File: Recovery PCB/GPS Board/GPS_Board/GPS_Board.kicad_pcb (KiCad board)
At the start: 2 copper layers, 85.7 x 50.8 mm, 11 parts, among them J1 XT30-M, J2 XT30-M, U1 Teensy4.1

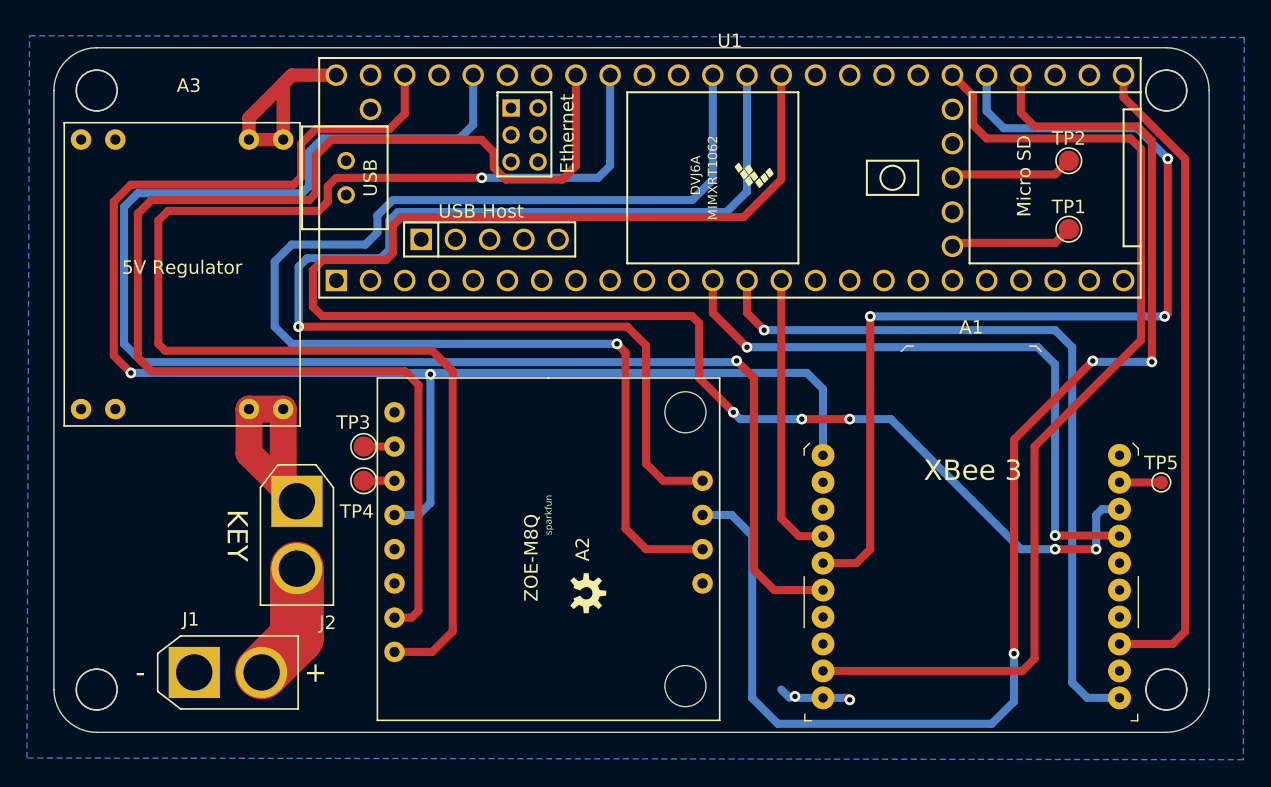
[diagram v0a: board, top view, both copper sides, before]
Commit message: Initial Board Layout
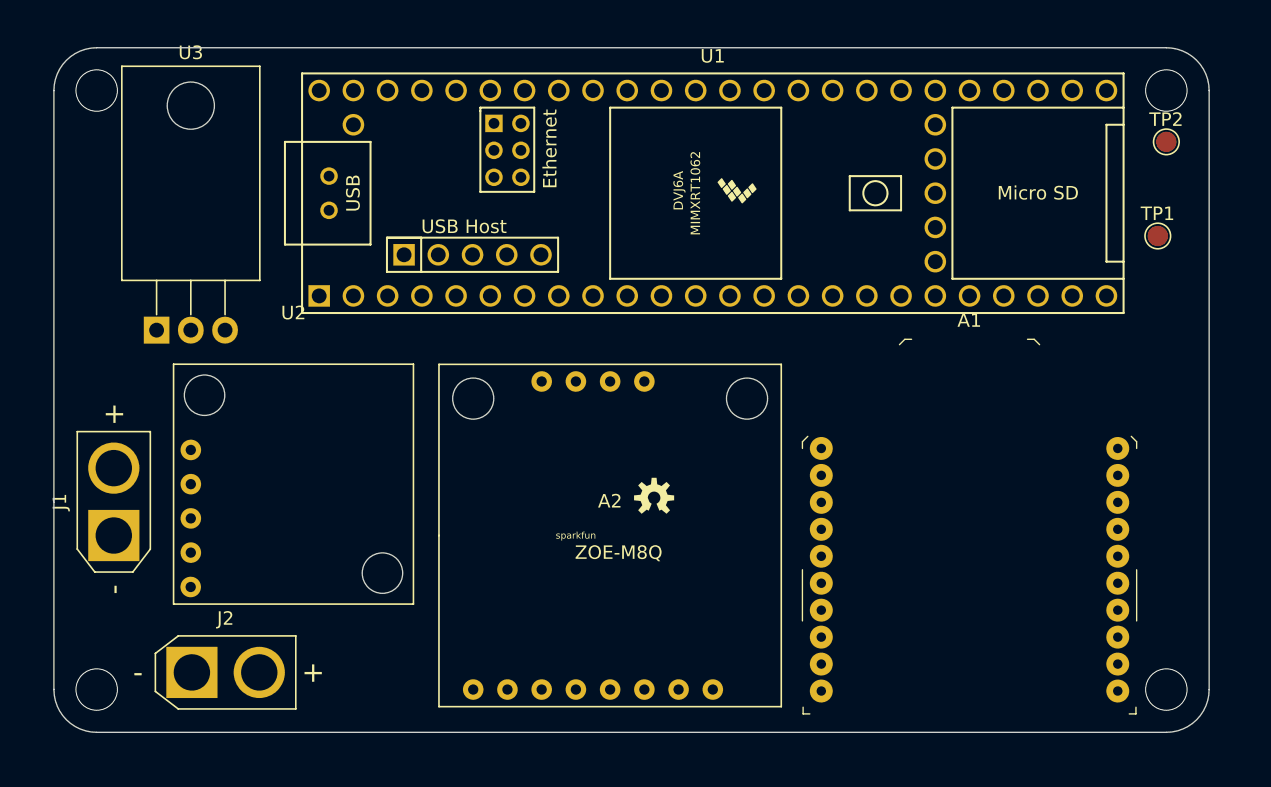
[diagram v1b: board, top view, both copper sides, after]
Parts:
- removed A3: Eboot-MP1584EN-5V-Power-Supply, GPS Board:EBOOT-MP1584EN-5N-POWER-SUPPLY
- removed TP3, TP4: TestPoint, TestPoint:TestPoint_Pad_D1.5mm
- removed TP5: TestPoint, TestPoint:TestPoint_Pad_D1.0mm
- added U2: D24V22F5_VoltageRegulator, GPS Board:D24V22F5_VoltageRegulator, F.Cu at (128.9, 92.7)
- added U3: LD1117v33, Package_TO_SOT_THT:TO-220-3_Horizontal_TabDown, F.Cu at (118.7, 81.3)
- moved J2 14.9 mm to (121.4, 106.7), turned to 0 degrees
- moved J1 11.8 mm to (115.6, 96.5), turned to 90 degrees
- moved TP2 7.37 mm to (193.7, 67.3)
- moved TP1 6.62 mm to (193.0, 74.3)
- moved A2 4.68 mm to (152.4, 96.5), turned to 0 degrees
- moved U1 1.71 mm to (160.0, 71.1)
- moved A1 0.52 mm to (179.1, 99.1)
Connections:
- net MOSI renamed /XBee_MOSI
- net Net-(A1-Pad13) renamed /XBEE_SLEEP
- net Net-(A1-Pad17) renamed /XBee_CS
- net Net-(A1-Pad18) renamed /XBee_SCK
- net Net-(A1-Pad4) renamed /XBee_MISO
- net Net-(A1-Pad6) renamed /XBee_PWM
- net Net-(A1-Pad9) renamed /XBee_DTR
- net Net-(A2-Pad7) renamed /GPS_SCL
- net Net-(A2-Pad8) renamed /GPS_SDA
- A1 pad 1: Net-(A1-Pad1) -> +3V3
- A1 pad 12: (no net) -> Net-(A1-Pad12)
- A1 pad 14: (no net) -> Net-(A1-Pad14)
- A1 pad 15: (no net) -> Net-(A1-Pad15)
- A1 pad 16: (no net) -> Net-(A1-Pad16)
- A1 pad 19: Net-(A1-Pad19) -> /XBEE_SCL
- A1 pad 2: (no net) -> /XBEE_TX
- A1 pad 20: (no net) -> Net-(A1-Pad20)
- A1 pad 3: (no net) -> /XBEE_RX
- A1 pad 5: Net-(A1-Pad5) -> /XBee_Reset
- A1 pad 7: (no net) -> /XBEE_SDA
- A1 pad 8: (no net) -> Net-(A1-Pad8)
- A2 pad 1: (no net) -> Net-(A2-Pad1)
- A2 pad 10: Net-(A2-Pad10) -> /GPS_PPS
- A2 pad 11: Net-(A2-Pad11) -> /GPS_RESET
- A2 pad 12: (no net) -> /GPS_INT
- A2 pad 2: Net-(A2-Pad2) -> /GPS_TX
- A2 pad 3: Net-(A2-Pad3) -> /GPS_RX
- A2 pad 4: Net-(A1-Pad1) -> +3V3
- A2 pad 5: (no net) -> Net-(A2-Pad5)
- U1 pad 10: (no net) -> Net-(U1-Pad10)
- U1 pad 11: (no net) -> Net-(U1-Pad11)
- U1 pad 15: (no net) -> +3V3
- U1 pad 16: (no net) -> Net-(U1-Pad16)
- U1 pad 17: (no net) -> Net-(U1-Pad17)
- U1 pad 18: (no net) -> Net-(U1-Pad18)
- U1 pad 19: (no net) -> Net-(U1-Pad19)
- U1 pad 2: (no net) -> /GPS_TX
- U1 pad 20: (no net) -> /XBEE_TX
- U1 pad 21: (no net) -> /XBEE_RX
- U1 pad 22: (no net) -> Net-(U1-Pad22)
- U1 pad 23: (no net) -> Net-(U1-Pad23)
- U1 pad 24: (no net) -> Net-(U1-Pad24)
- U1 pad 26: (no net) -> Net-(U1-Pad26)
- U1 pad 27: (no net) -> Net-(U1-Pad27)
- U1 pad 28: Net-(A2-Pad10) -> /GPS_RESET
- U1 pad 29: Net-(A1-Pad5) -> /XBee_RESET
- U1 pad 3: (no net) -> /GPS_RX
- U1 pad 31: (no net) -> Net-(U1-Pad31)
- U1 pad 32: (no net) -> Net-(U1-Pad32)
- U1 pad 33: (no net) -> Net-(U1-Pad33)
- U1 pad 36: Net-(A2-Pad9) -> /GPS_INT
- U1 pad 37: Net-(A2-Pad11) -> /GPS_PPS
- U1 pad 38: (no net) -> /XBEE_SCL
- U1 pad 39: (no net) -> /XBEE_SDA
- U1 pad 4: (no net) -> Net-(U1-Pad4)
- U1 pad 42: (no net) -> Net-(U1-Pad42)
- U1 pad 43: (no net) -> Net-(U1-Pad43)
- U1 pad 45: (no net) -> Net-(U1-Pad45)
- U1 pad 46: Net-(A1-Pad1) -> +3V3
- U1 pad 49: (no net) -> Net-(U1-Pad49)
- U1 pad 5: (no net) -> Net-(U1-Pad5)
- U1 pad 51: (no net) -> +3V3
- U1 pad 53: (no net) -> Net-(U1-Pad53)
- U1 pad 54: (no net) -> Net-(U1-Pad54)
- U1 pad 55: (no net) -> +5V
- U1 pad 56: (no net) -> Net-(U1-Pad56)
- U1 pad 57: (no net) -> Net-(U1-Pad57)
- U1 pad 58: (no net) -> GND
- U1 pad 59: (no net) -> GND
- U1 pad 6: (no net) -> Net-(U1-Pad6)
- U1 pad 60: (no net) -> Net-(U1-Pad60)
- U1 pad 61: (no net) -> Net-(U1-Pad61)
- U1 pad 62: (no net) -> Net-(U1-Pad62)
- U1 pad 63: (no net) -> Net-(U1-Pad63)
- U1 pad 64: (no net) -> GND
- U1 pad 65: (no net) -> Net-(U1-Pad65)
- U1 pad 66: (no net) -> Net-(U1-Pad66)
- U1 pad 67: (no net) -> Net-(U1-Pad67)
- U1 pad 7: (no net) -> Net-(U1-Pad7)
- U1 pad 8: (no net) -> Net-(U1-Pad8)
- U1 pad 9: (no net) -> Net-(U1-Pad9)
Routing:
- net /XBee_SCK: track 121.6 -> 0.00 mm, vias 5 -> 0
- net /XBee_PWM: track 111.6 -> 0.00 mm, vias 1 -> 0
- net Net-(A1-Pad1): track 111.2 -> 0.00 mm, vias 2 -> 0
- net Net-(A2-Pad10): track 99.2 -> 0.00 mm, vias 3 -> 0
- net /GPS_SDA: track 98.7 -> 0.00 mm, vias 1 -> 0
- net /GPS_SCL: track 96.6 -> 0.00 mm
- net Net-(A2-Pad11): track 94.6 -> 0.00 mm, vias 1 -> 0
- net Net-(A2-Pad9): track 89.8 -> 0.00 mm, vias 1 -> 0
- net /XBee_DTR: track 74.7 -> 0.00 mm
- net Net-(A1-Pad5): track 72.4 -> 0.00 mm, vias 3 -> 0
- net /XBee_MOSI: track 56.5 -> 0.00 mm, vias 1 -> 0
- net /XBEE_SLEEP: track 48.4 -> 0.00 mm
- net /XBee_CS: track 46.9 -> 0.00 mm, vias 2 -> 0
- net /XBee_MISO: track 21.3 -> 0.00 mm
- net Net-(J2-Pad1): track 18.1 -> 0.00 mm
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- removed copper zone on B.Cu, net GND
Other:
- outline, holes or cut-outs redrawn
- board text removed: "Created By: Bryce D. Ashley J."
- board text removed: "JLCJLCJLCJLC"
- board text removed: "KEY"
- board text removed: "XBee 3"
